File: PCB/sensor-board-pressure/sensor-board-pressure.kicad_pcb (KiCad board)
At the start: 2 copper layers, 23.6 x 23.5 mm, 10 parts, among them U1 MAGNETIC POGO CONN., U2 MAGNETIC POGO CONN.

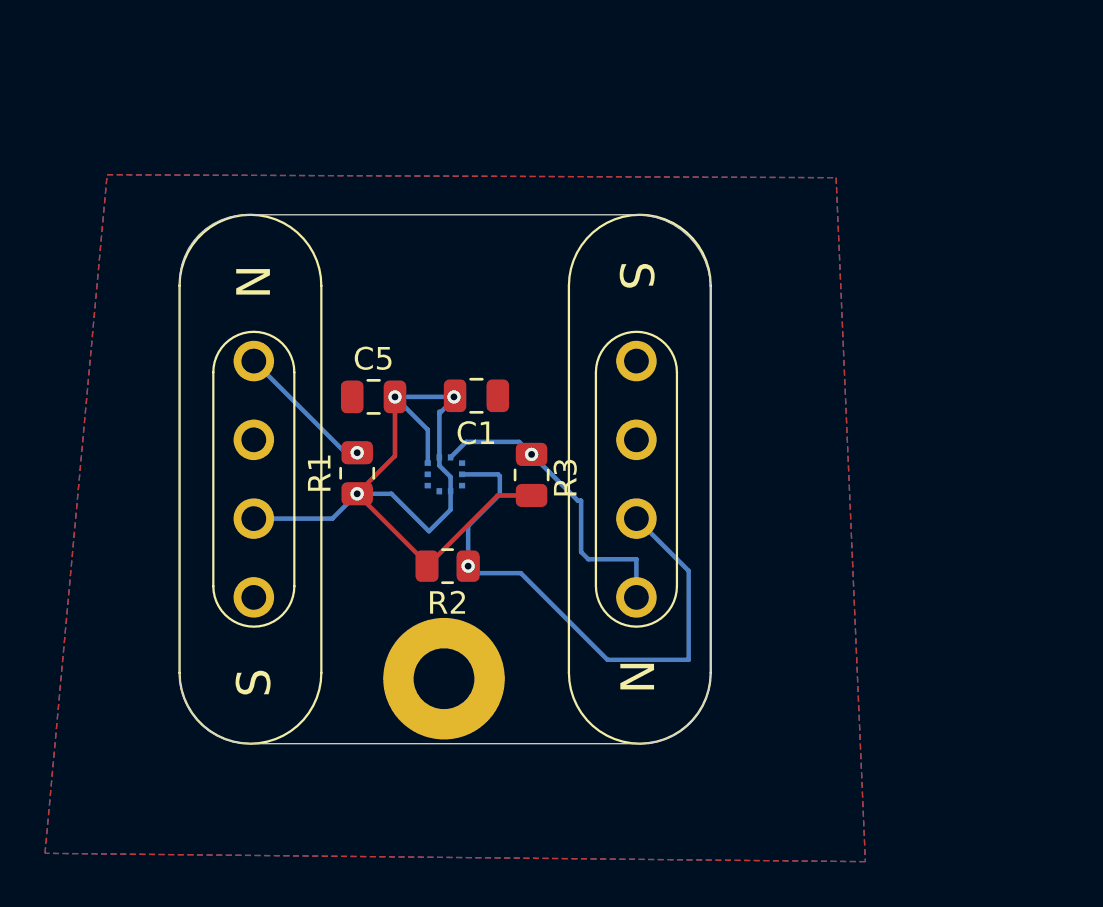
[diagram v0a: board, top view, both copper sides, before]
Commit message: made some changes
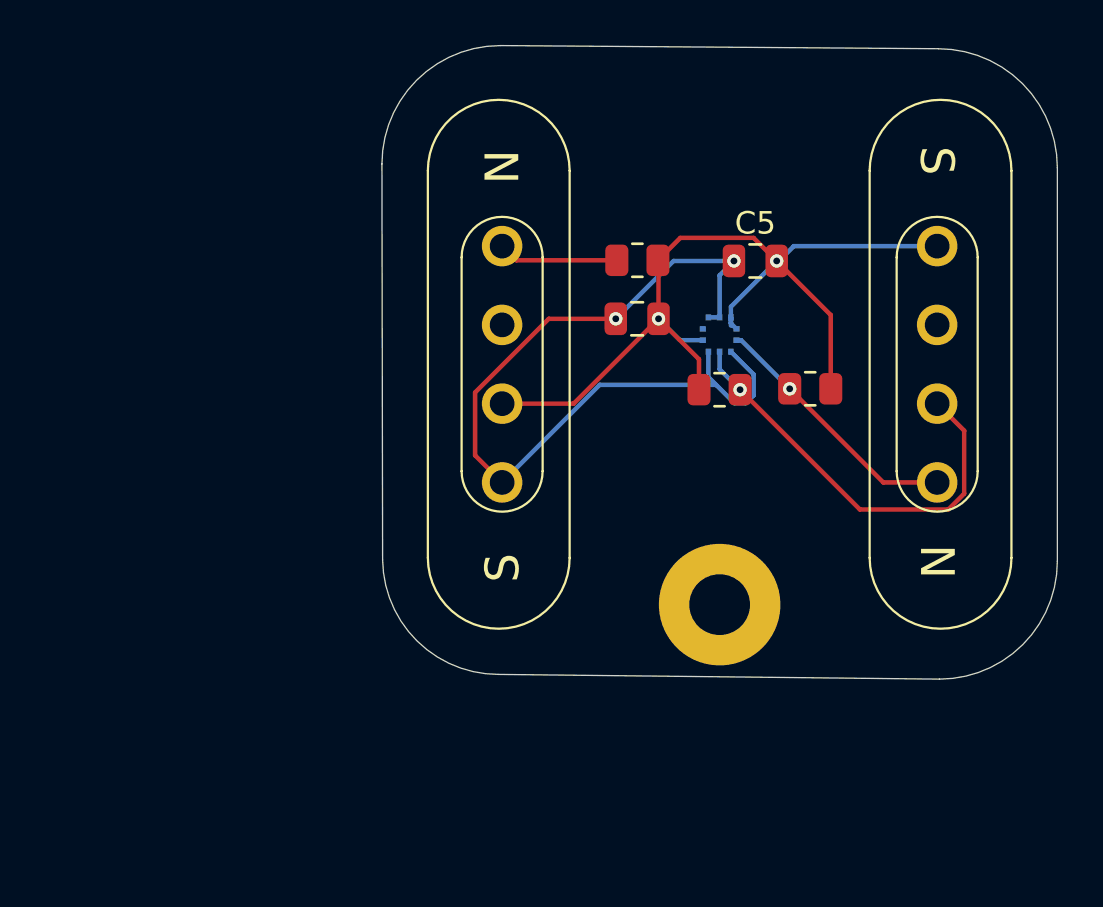
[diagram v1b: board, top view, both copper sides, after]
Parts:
- moved C5 18.0 mm to (113.1, 56.2)
- moved R1 15.6 mm to (107.9, 56.2), turned to 180 degrees
- moved R2 14.4 mm to (111.5, 61.9)
- moved U1 14.3 mm to (121.2, 60.8)
- moved BMP390 13.7 mm to (111.5, 59.5), turned to 90 degrees
- moved R3 13.0 mm to (115.5, 61.9), turned to 0 degrees
- moved H1 12.7 mm to (111.5, 71.5)
- moved G*** 12.7 mm to (111.5, 65.4)
- moved U2 12.2 mm to (101.8, 60.8)
- moved C1 7.92 mm to (107.8, 58.8), turned to 0 degrees
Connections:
- U1 pad 1: unconnected-(U1-Pad1) -> +3.3V
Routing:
- net GND: track 0.00 -> 39.1 mm, vias 0 -> 2
- net /SDA: track 25.1 -> 19.0 mm
- net +3.3V: track 37.5 -> 41.9 mm, vias 3 -> 2
- net /SCL: track 13.7 -> 11.5 mm
- net /ID: track 6.50 -> 5.36 mm, vias 1 -> 0
- removed copper zone on B.Cu, net GND
- removed copper zone on F.Cu, net GND
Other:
- board size 23.6 x 23.5 mm -> 30 x 28.1 mm
- board text added: "Barometer"
- board text removed: "BAROMETER"
